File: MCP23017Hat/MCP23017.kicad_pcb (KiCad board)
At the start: 2 copper layers, 65 x 56 mm, 12 parts, among them J0 RPi_GPIO, J1 Address Jumper, T1 GP0, T2 GP1, U1 MCP23017

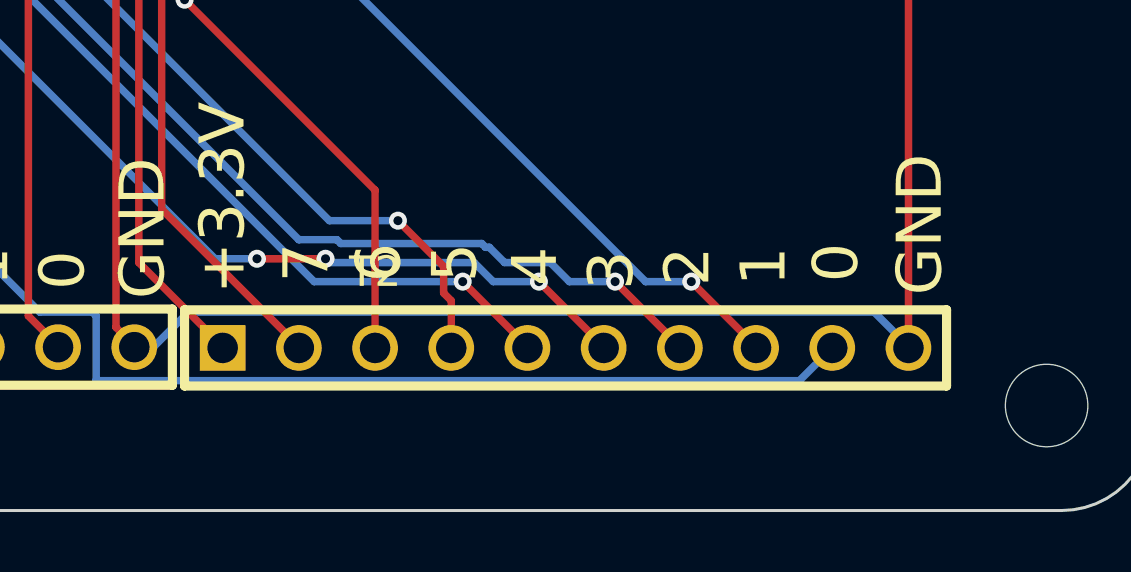
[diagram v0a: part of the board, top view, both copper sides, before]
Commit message: Minor updates
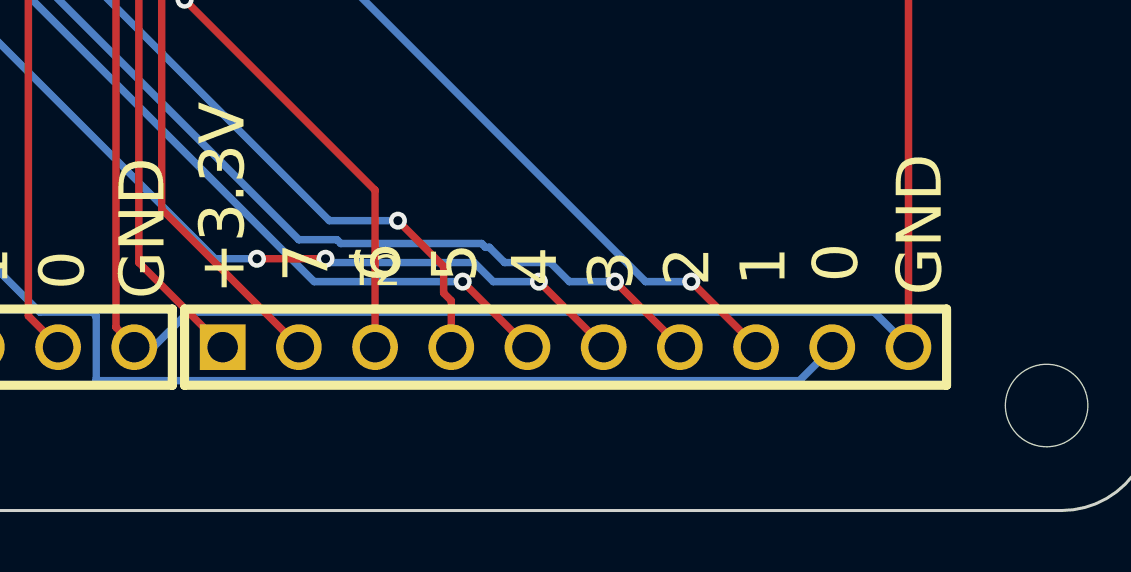
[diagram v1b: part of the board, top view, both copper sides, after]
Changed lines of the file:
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@@
   )
   (module ScrewTerm_2.54-10 (layer F.Cu)
-    (at 77.216 82.4738)
+    (at 77.216 82.4484)
     (descr "Screw Terminals, 2.54 pitch, 10 position")
     (tags CONN)
